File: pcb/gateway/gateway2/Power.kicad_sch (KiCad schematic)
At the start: 12 parts, among them U3 RT6150AGQW

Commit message: Doing some routing.
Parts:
- L5: footprint Richtek_RT6150:WDFN-10-1EP_3x3mm_P0.5mm_EP1.8x2.5mm -> Abracon_AOTA_B201610S:L_0806_2016Metric
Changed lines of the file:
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@@
 			)
 		)
-		(property "Footprint" "Richtek_RT6150:WDFN-10-1EP_3x3mm_P0.5mm_EP1.8x2.5mm"
+		(property "Footprint" "Abracon_AOTA_B201610S:L_0806_2016Metric"
 			(at 203.2 95.25 0)
 			(hide yes)

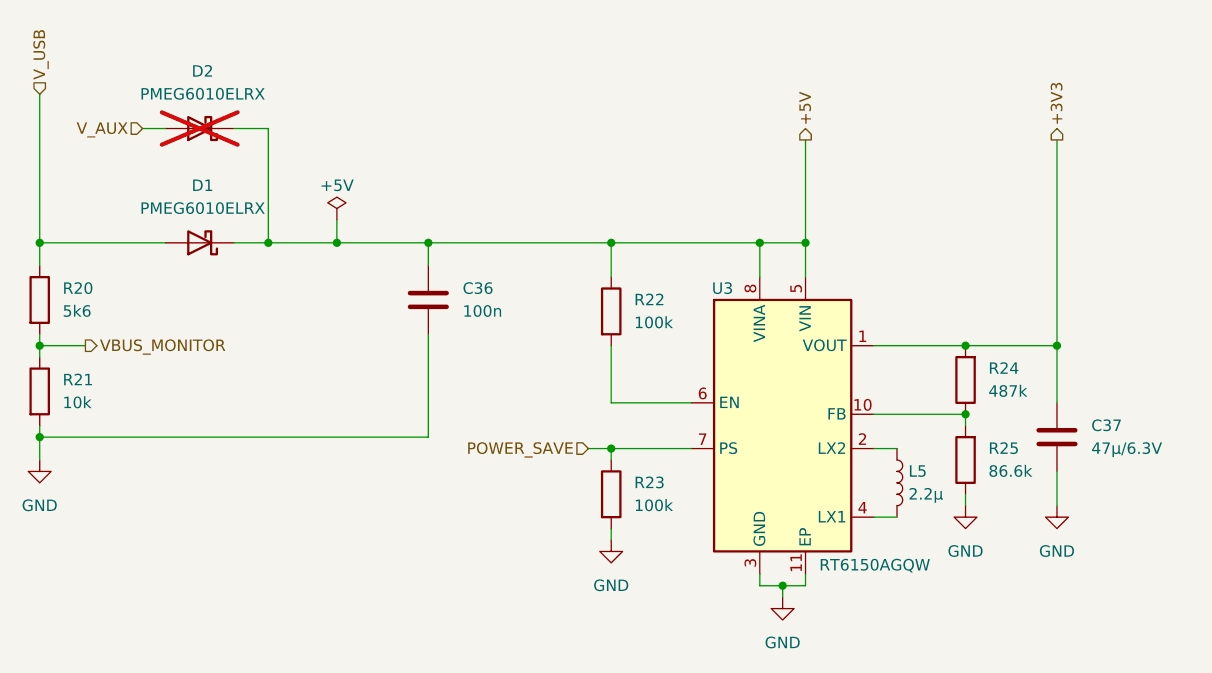
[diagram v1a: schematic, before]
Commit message: Moving stuff to proper library.
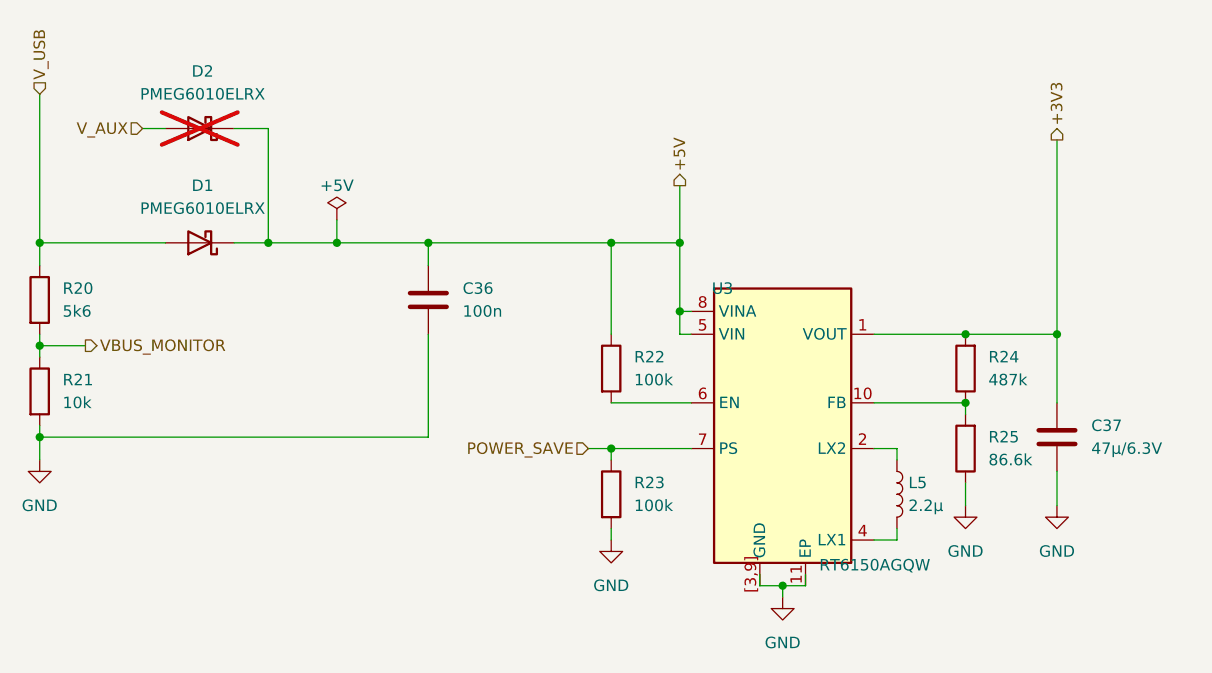
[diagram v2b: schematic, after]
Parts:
- U3: footprint Richtek_RT6150:WDFN-10-1EP_3x3mm_P0.5mm_EP1.8x2.5mm -> Package_DFN_QFN:WDFN-10-1EP_3x3mm_P0.5mm_EP1.8x2.5mm; symbol Richtek_RT6150:RT6150AGQW -> Regulator_Switching:RT6150AGQW
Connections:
- net GND: now also U3.[3,9] (GND); no longer U3.3 (GND), U3.9 (GND)
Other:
- moved on the sheet: L5, R22, R24, R25, U3
